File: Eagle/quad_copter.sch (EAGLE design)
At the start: 12 parts, among them X1 STM32F4_DISC

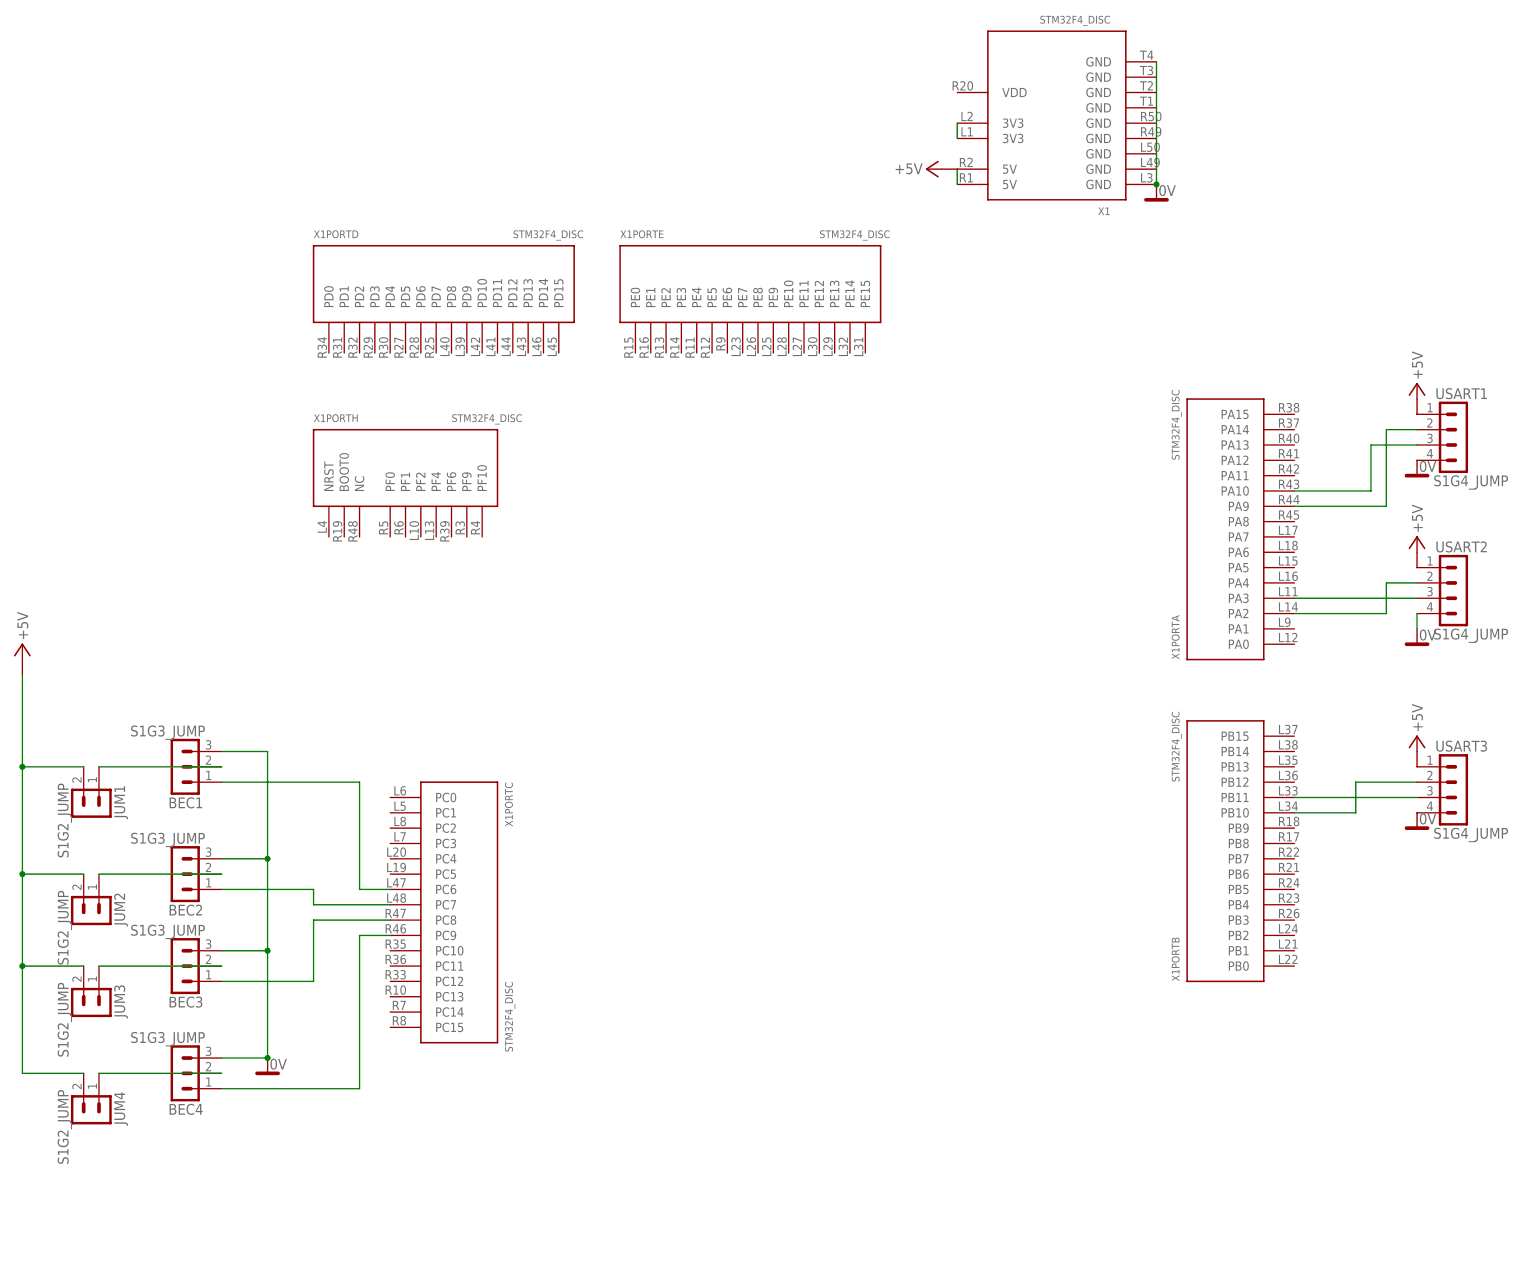
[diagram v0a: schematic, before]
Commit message: new scheme and board
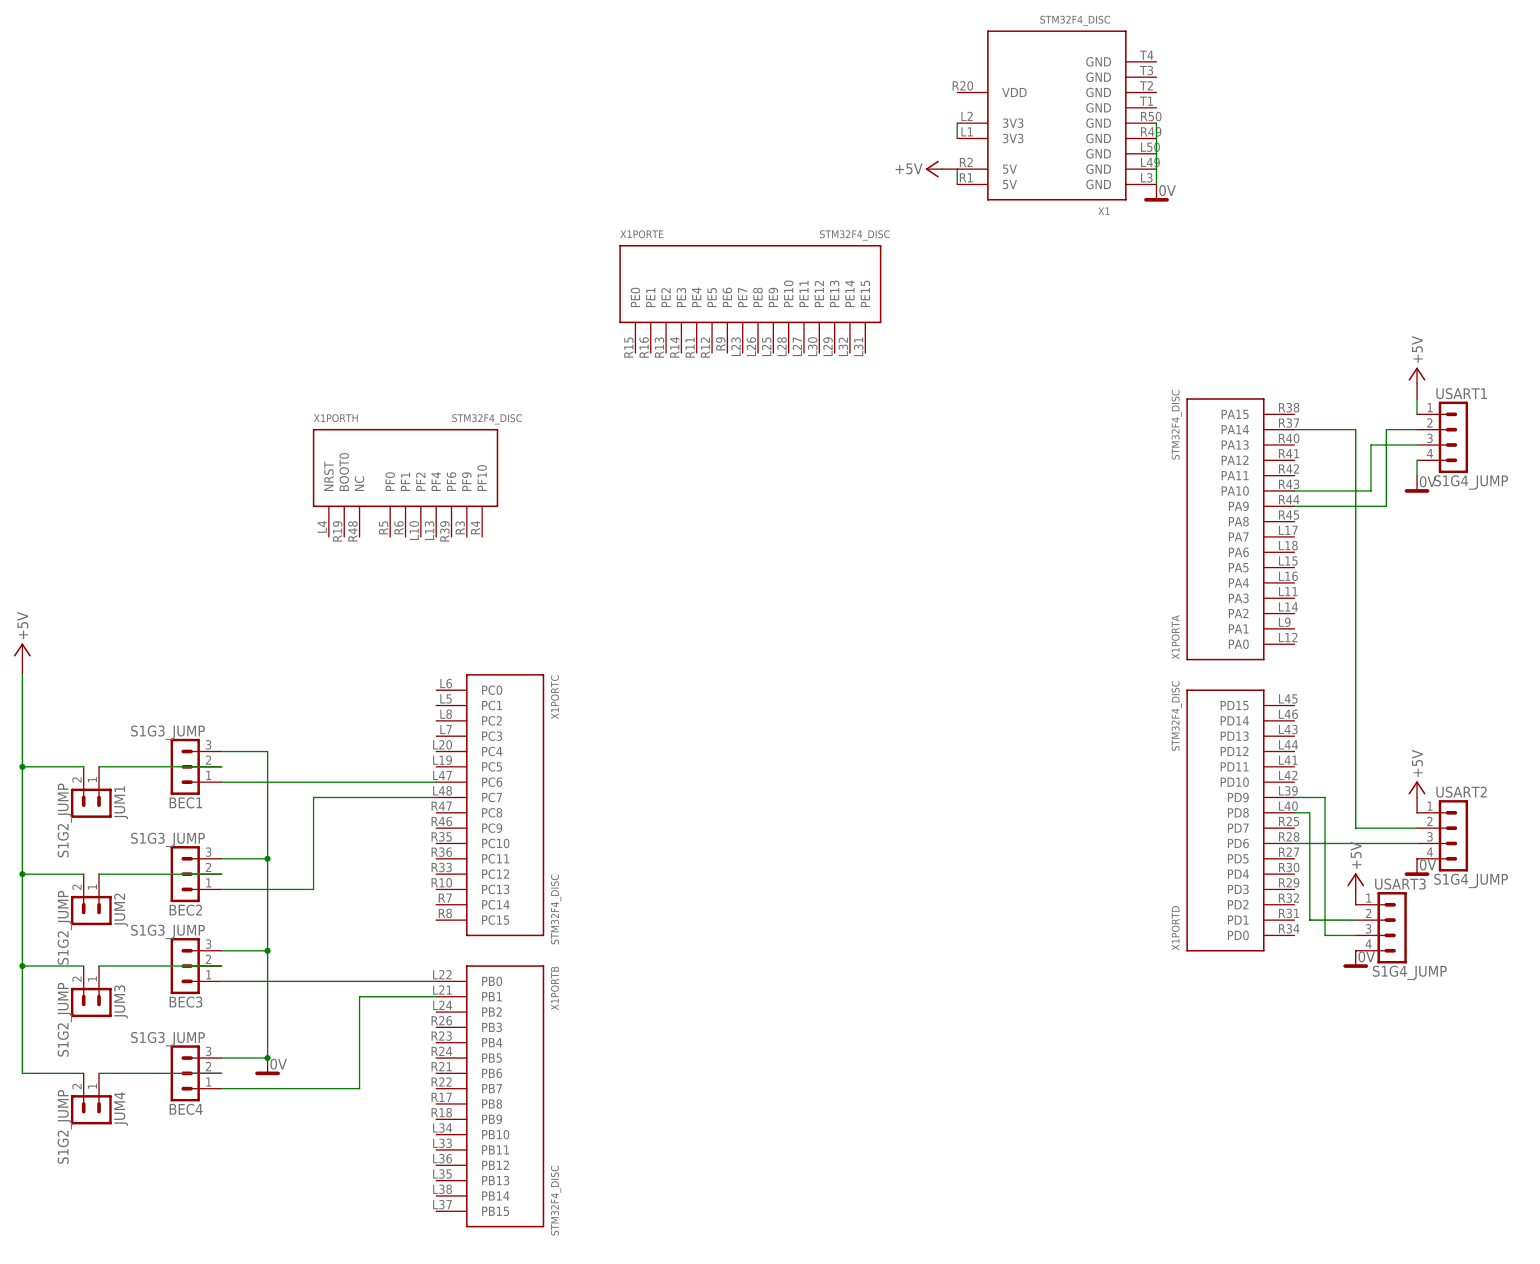
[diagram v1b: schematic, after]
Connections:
- removed net N$6: USART3.3, X1PORTB.PB11
- new net N$13: USART2.3, X1PORTD.PD6
- net 0V: now also X1PWR.GND@2, X1PWR.GND@3, X1PWR.GND@4, X1PWR.GND@5; no longer X1PWR.GND@9
- net N$1: now also USART3.3, X1PORTD.PD9; no longer USART2.2, X1PORTA.PA2
- net N$14: now also X1PORTB.PB1; no longer X1PORTC.PC9
- net N$15: now also X1PORTB.PB0; no longer X1PORTC.PC8
- net N$2: now also USART3.2, X1PORTD.PD8; no longer USART2.3, X1PORTA.PA3
- net N$5: now also USART2.2, X1PORTA.PA14; no longer USART3.2, X1PORTB.PB10
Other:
- moved on the sheet: USART2, USART3, X1PORTB, X1PORTC, X1PORTD
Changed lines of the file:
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@@
 <parts>
 <part name="X1" library="stm32f3_disc" deviceset="STM32F4_DISC" device=""/>
+<part name="USART1" library="#PaJa_konektory" deviceset="S1G4_JUMP" device=""/>
 <part name="USART2" library="#PaJa_konektory" deviceset="S1G4_JUMP" device=""/>
-<part name="NAP1" library="#PaJa_30" deviceset="+5V" device=""/>
-<part name="0V1" library="#PaJa_30" deviceset="0V" device=""/>
-<part name="USART1" library="#PaJa_konektory" deviceset="S1G4_JUMP" device=""/>
-<part name="USART3" library="#PaJa_konektory" deviceset="S1G4_JUMP" device=""/>
 <part name="0V2" library="#PaJa_30" deviceset="0V" device=""/>
 <part name="0V3" library="#PaJa_30" deviceset="0V" device=""/>
@@
 <part name="NAP5" library="#PaJa_30" deviceset="+5V" device=""/>
 <part name="0V5" library="#PaJa_30" deviceset="0V" device=""/>
+<part name="USART3" library="#PaJa_konektory" deviceset="S1G4_JUMP" device=""/>
+<part name="0V1" library="#PaJa_30" deviceset="0V" device=""/>
+<part name="NAP1" library="#PaJa_30" deviceset="+5V" device=""/>
 </parts>
 <sheets>
@@
 <instance part="X1" gate="PWR" x="106.68" y="81.28" rot="R90"/>
 <instance part="X1" gate="PORTA" x="134.62" y="10.16" rot="R90"/>
-<instance part="X1" gate="PORTB" x="134.62" y="-43.18" rot="R90"/>
-<instance part="X1" gate="PORTC" x="5.08" y="-50.8" rot="R270"/>
-<instance part="X1" gate="PORTD" x="2.54" y="50.8"/>
+<instance part="X1" gate="PORTB" x="12.7" y="-81.28" rot="R270"/>
+<instance part="X1" gate="PORTC" x="12.7" y="-33.02" rot="R270"/>
+<instance part="X1" gate="PORTD" x="134.62" y="-38.1" rot="R90"/>
 <instance part="X1" gate="PORTE" x="53.34" y="50.8"/>
 <instance part="X1" gate="PORTH" x="-2.54" y="20.32"/>
-<instance part="USART2" gate="JUMP" x="167.64" y="2.54" rot="R270"/>
-<instance part="NAP1" gate="+5" x="165.1" y="10.16"/>
-<instance part="0V1" gate="0" x="165.1" y="-7.62"/>
 <instance part="USART1" gate="JUMP" x="167.64" y="27.94" rot="R270"/>
-<instance part="USART3" gate="JUMP" x="167.64" y="-30.48" rot="R270"/>
-<instance part="0V2" gate="0" x="165.1" y="-38.1"/>
-<instance part="0V3" gate="0" x="165.1" y="20.32"/>
-<instance part="NAP2" gate="+5" x="165.1" y="35.56"/>
-<instance part="NAP3" gate="+5" x="165.1" y="-22.86"/>
+<instance part="USART2" gate="JUMP" x="167.64" y="-38.1" rot="R270"/>
+<instance part="0V2" gate="0" x="165.1" y="-45.72"/>
+<instance part="0V3" gate="0" x="165.1" y="17.78"/>
+<instance part="NAP2" gate="+5" x="165.1" y="38.1"/>
+<instance part="NAP3" gate="+5" x="165.1" y="-30.48"/>
 <instance part="NAP4" gate="+5" x="83.82" y="71.12" rot="R90"/>
 <instance part="0V4" gate="0" x="121.92" y="66.04"/>
@@
 <instance part="NAP5" gate="+5" x="-66.04" y="-7.62"/>
 <instance part="0V5" gate="0" x="-25.4" y="-78.74"/>
+<instance part="USART3" gate="JUMP" x="157.48" y="-53.34" rot="R270"/>
+<instance part="0V1" gate="0" x="154.94" y="-60.96"/>
+<instance part="NAP1" gate="+5" x="154.94" y="-45.72"/>
 </instances>
 <busses>
 </busses>
 <nets>
-<net name="N$1" class="0">
-<segment>
-<pinref part="X1" gate="PORTA" pin="PA2"/>
-<wire x1="144.78" y1="-2.54" x2="160.02" y2="-2.54" width="0.1524" layer="91"/>
-<wire x1="160.02" y1="-2.54" x2="160.02" y2="2.54" width="0.1524" layer="91"/>
-<wire x1="160.02" y1="2.54" x2="165.1" y2="2.54" width="0.1524" layer="91"/>
-<pinref part="USART2" gate="JUMP" pin="2"/>
-</segment>
-</net>
-<net name="N$2" class="0">
-<segment>
-<pinref part="X1" gate="PORTA" pin="PA3"/>
-<wire x1="144.78" y1="0" x2="165.1" y2="0" width="0.1524" layer="91"/>
-<pinref part="USART2" gate="JUMP" pin="3"/>
-</segment>
-</net>
 <net name="+5V" class="0">
-<segment>
-<pinref part="USART2" gate="JUMP" pin="1"/>
-<pinref part="NAP1" gate="+5" pin="+5V"/>
-</segment>
 <segment>
 <pinref part="USART1" gate="JUMP" pin="1"/>
 <pinref part="NAP2" gate="+5" pin="+5V"/>
-</segment>
-<segment>
-<pinref part="USART3" gate="JUMP" pin="1"/>
+<wire x1="165.1" y1="33.02" x2="165.1" y2="30.48" width="0.1524" layer="91"/>
+</segment>
+<segment>
+<pinref part="USART2" gate="JUMP" pin="1"/>
 <pinref part="NAP3" gate="+5" pin="+5V"/>
 </segment>
@@
 <junction x="-66.04" y="-27.94"/>
 </segment>
+<segment>
+<pinref part="USART3" gate="JUMP" pin="1"/>
+<pinref part="NAP1" gate="+5" pin="+5V"/>
+</segment>
 </net>
 <net name="0V" class="0">
 <segment>
 <pinref part="USART2" gate="JUMP" pin="4"/>
-<pinref part="0V1" gate="0" pin="0V"/>
-<wire x1="165.1" y1="-2.54" x2="165.1" y2="-5.08" width="0.1524" layer="91"/>
-</segment>
-<segment>
-<pinref part="USART3" gate="JUMP" pin="4"/>
 <pinref part="0V2" gate="0" pin="0V"/>
 </segment>
@@
 <pinref part="USART1" gate="JUMP" pin="4"/>
 <pinref part="0V3" gate="0" pin="0V"/>
+<wire x1="165.1" y1="20.32" x2="165.1" y2="22.86" width="0.1524" layer="91"/>
 </segment>
 <segment>
 <pinref part="X1" gate="PWR" pin="GND@1"/>
-<pinref part="X1" gate="PWR" pin="GND@9"/>
-<wire x1="121.92" y1="68.58" x2="121.92" y2="88.9" width="0.1524" layer="91"/>
 <pinref part="0V4" gate="0" pin="0V"/>
-<junction x="121.92" y="68.58"/>
+<pinref part="X1" gate="PWR" pin="GND@3"/>
+<pinref part="X1" gate="PWR" pin="GND@2"/>
+<wire x1="121.92" y1="68.58" x2="121.92" y2="71.12" width="0.1524" layer="91"/>
+<wire x1="121.92" y1="71.12" x2="121.92" y2="73.66" width="0.1524" layer="91"/>
+<pinref part="X1" gate="PWR" pin="GND@4"/>
+<pinref part="X1" gate="PWR" pin="GND@5"/>
+<wire x1="121.92" y1="76.2" x2="121.92" y2="78.74" width="0.1524" layer="91"/>
+<wire x1="121.92" y1="73.66" x2="121.92" y2="76.2" width="0.1524" layer="91"/>
 </segment>
 <segment>
@@
 <junction x="-25.4" y="-43.18"/>
 </segment>
+<segment>
+<pinref part="USART3" gate="JUMP" pin="4"/>
+<pinref part="0V1" gate="0" pin="0V"/>
+</segment>
 </net>
 <net name="N$3" class="0">
@@
 </segment>
 </net>
-<net name="N$5" class="0">
-<segment>
-<pinref part="X1" gate="PORTB" pin="PB10"/>
-<wire x1="144.78" y1="-35.56" x2="154.94" y2="-35.56" width="0.1524" layer="91"/>
-<wire x1="154.94" y1="-35.56" x2="154.94" y2="-30.48" width="0.1524" layer="91"/>
-<pinref part="USART3" gate="JUMP" pin="2"/>
-<wire x1="154.94" y1="-30.48" x2="165.1" y2="-30.48" width="0.1524" layer="91"/>
-</segment>
-</net>
-<net name="N$6" class="0">
-<segment>
-<pinref part="X1" gate="PORTB" pin="PB11"/>
-<wire x1="144.78" y1="-33.02" x2="165.1" y2="-33.02" width="0.1524" layer="91"/>
-<pinref part="USART3" gate="JUMP" pin="3"/>
-</segment>
-</net>
 <net name="N$7" class="0">
 <segment>
@@
 <pinref part="BEC4" gate="JUMP" pin="1"/>
 <wire x1="-33.02" y1="-81.28" x2="-10.16" y2="-81.28" width="0.1524" layer="91"/>
-<wire x1="-10.16" y1="-81.28" x2="-10.16" y2="-55.88" width="0.1524" layer="91"/>
-<pinref part="X1" gate="PORTC" pin="PC9"/>
-<wire x1="-10.16" y1="-55.88" x2="-5.08" y2="-55.88" width="0.1524" layer="91"/>
+<wire x1="-10.16" y1="-81.28" x2="-10.16" y2="-66.04" width="0.1524" layer="91"/>
+<pinref part="X1" gate="PORTB" pin="PB1"/>
+<wire x1="-10.16" y1="-66.04" x2="2.54" y2="-66.04" width="0.1524" layer="91"/>
 </segment>
 </net>
@@
 <segment>
 <pinref part="BEC3" gate="JUMP" pin="1"/>
-<wire x1="-33.02" y1="-63.5" x2="-17.78" y2="-63.5" width="0.1524" layer="91"/>
-<wire x1="-17.78" y1="-63.5" x2="-17.78" y2="-53.34" width="0.1524" layer="91"/>
-<pinref part="X1" gate="PORTC" pin="PC8"/>
-<wire x1="-17.78" y1="-53.34" x2="-5.08" y2="-53.34" width="0.1524" layer="91"/>
+<pinref part="X1" gate="PORTB" pin="PB0"/>
+<wire x1="-33.02" y1="-63.5" x2="2.54" y2="-63.5" width="0.1524" layer="91"/>
 </segment>
 </net>
@@
 <pinref part="BEC2" gate="JUMP" pin="1"/>
 <wire x1="-33.02" y1="-48.26" x2="-17.78" y2="-48.26" width="0.1524" layer="91"/>
-<wire x1="-17.78" y1="-48.26" x2="-17.78" y2="-50.8" width="0.1524" layer="91"/>
+<wire x1="-17.78" y1="-48.26" x2="-17.78" y2="-33.02" width="0.1524" layer="91"/>
 <pinref part="X1" gate="PORTC" pin="PC7"/>
-<wire x1="-17.78" y1="-50.8" x2="-5.08" y2="-50.8" width="0.1524" layer="91"/>
+<wire x1="-17.78" y1="-33.02" x2="2.54" y2="-33.02" width="0.1524" layer="91"/>
 </segment>
 </net>
@@
 <segment>
 <pinref part="BEC1" gate="JUMP" pin="1"/>
-<wire x1="-33.02" y1="-30.48" x2="-10.16" y2="-30.48" width="0.1524" layer="91"/>
-<wire x1="-10.16" y1="-30.48" x2="-10.16" y2="-48.26" width="0.1524" layer="91"/>
+<wire x1="-33.02" y1="-30.48" x2="2.54" y2="-30.48" width="0.1524" layer="91"/>
 <pinref part="X1" gate="PORTC" pin="PC6"/>
-<wire x1="-10.16" y1="-48.26" x2="-5.08" y2="-48.26" width="0.1524" layer="91"/>
-</segment>
-</net>
+</segment>
+</net>
+<net name="N$5" class="0">
+<segment>
+<pinref part="USART2" gate="JUMP" pin="2"/>
+<wire x1="165.1" y1="-38.1" x2="154.94" y2="-38.1" width="0.1524" layer="91"/>
+<wire x1="154.94" y1="-38.1" x2="154.94" y2="27.94" width="0.1524" layer="91"/>
+<pinref part="X1" gate="PORTA" pin="PA14"/>
+<wire x1="154.94" y1="27.94" x2="144.78" y2="27.94" width="0.1524" layer="91"/>
+</segment>
+</net>
+<net name="N$13" class="0">
+<segment>
+<pinref part="USART2" gate="JUMP" pin="3"/>
+<pinref part="X1" gate="PORTD" pin="PD6"/>
+<wire x1="165.1" y1="-40.64" x2="144.78" y2="-40.64" width="0.1524" layer="91"/>
+</segment>
+</net>
+<net name="N$1" class="0">
+<segment>
+<pinref part="X1" gate="PORTD" pin="PD9"/>
+<wire x1="144.78" y1="-33.02" x2="149.86" y2="-33.02" width="0.1524" layer="91"/>
+<wire x1="149.86" y1="-33.02" x2="149.86" y2="-55.88" width="0.1524" layer="91"/>
+<pinref part="USART3" gate="JUMP" pin="3"/>
+<wire x1="149.86" y1="-55.88" x2="154.94" y2="-55.88" width="0.1524" layer="91"/>
+</segment>
+</net>
+<net name="N$2" class="0">
+<segment>
+<pinref part="USART3" gate="JUMP" pin="2"/>
+<wire x1="154.94" y1="-53.34" x2="147.32" y2="-53.34" width="0.1524" layer="91"/>
+<wire x1="147.32" y1="-53.34" x2="147.32" y2="-35.56" width="0.1524" layer="91"/>
+<pinref part="X1" gate="PORTD" pin="PD8"/>
+<wire x1="147.32" y1="-35.56" x2="144.78" y2="-35.56" width="0.1524" layer="91"/>
+</segment>
+</net>
